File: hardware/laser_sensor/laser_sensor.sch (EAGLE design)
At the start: 11 parts, among them IC1 NE555D, J1 B4B-XH-A(LF)(SN)

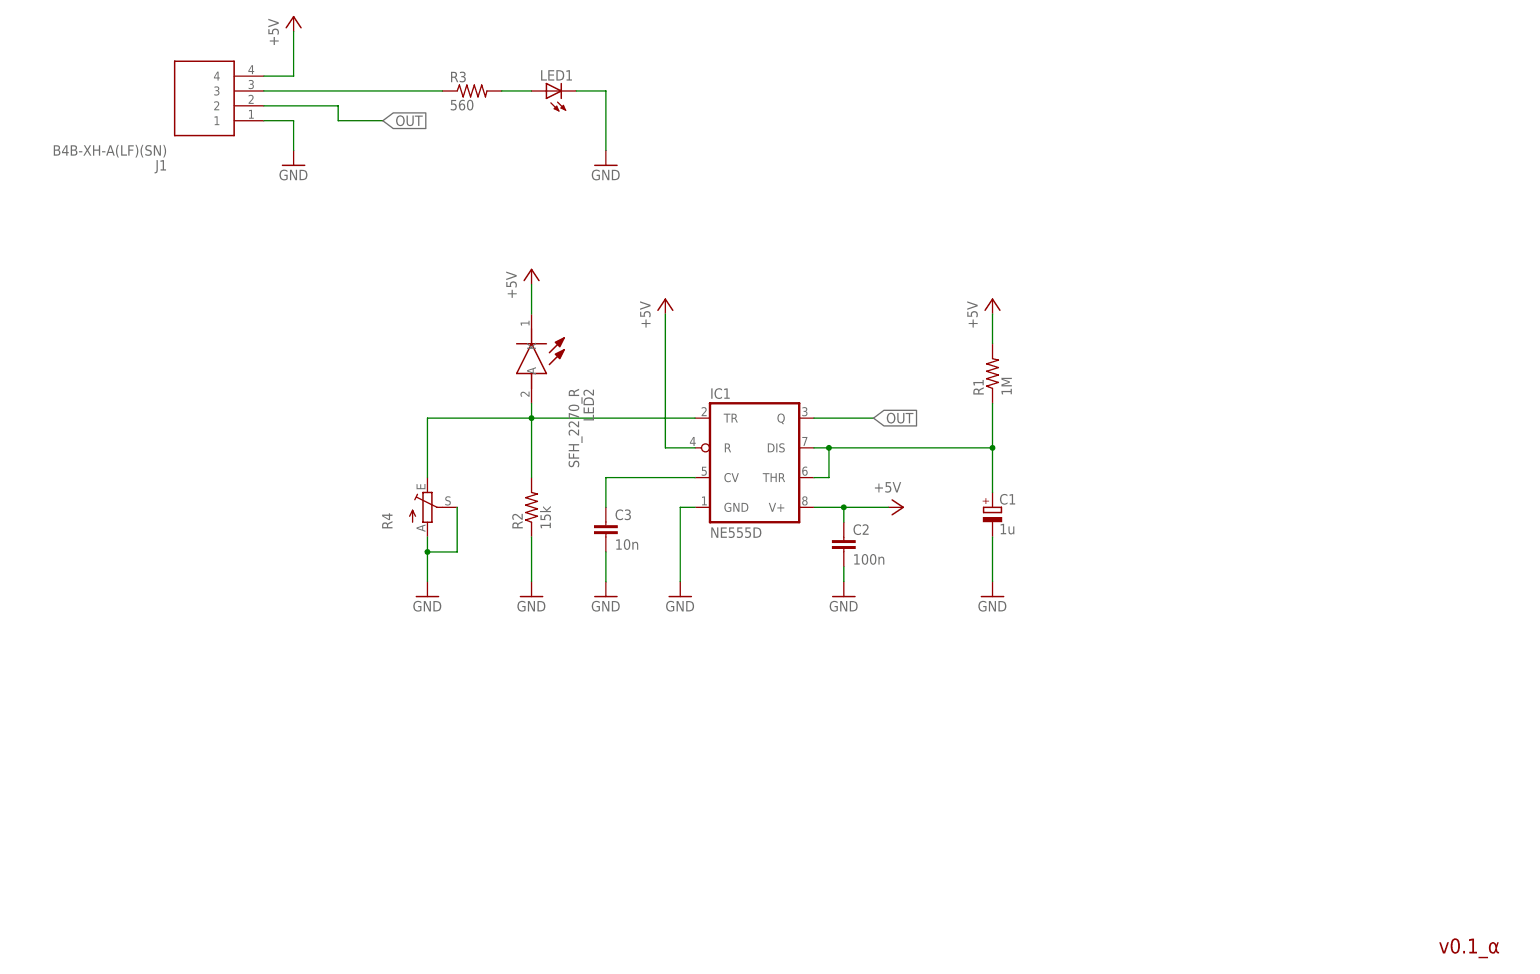
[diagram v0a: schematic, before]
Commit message: sensor redesign
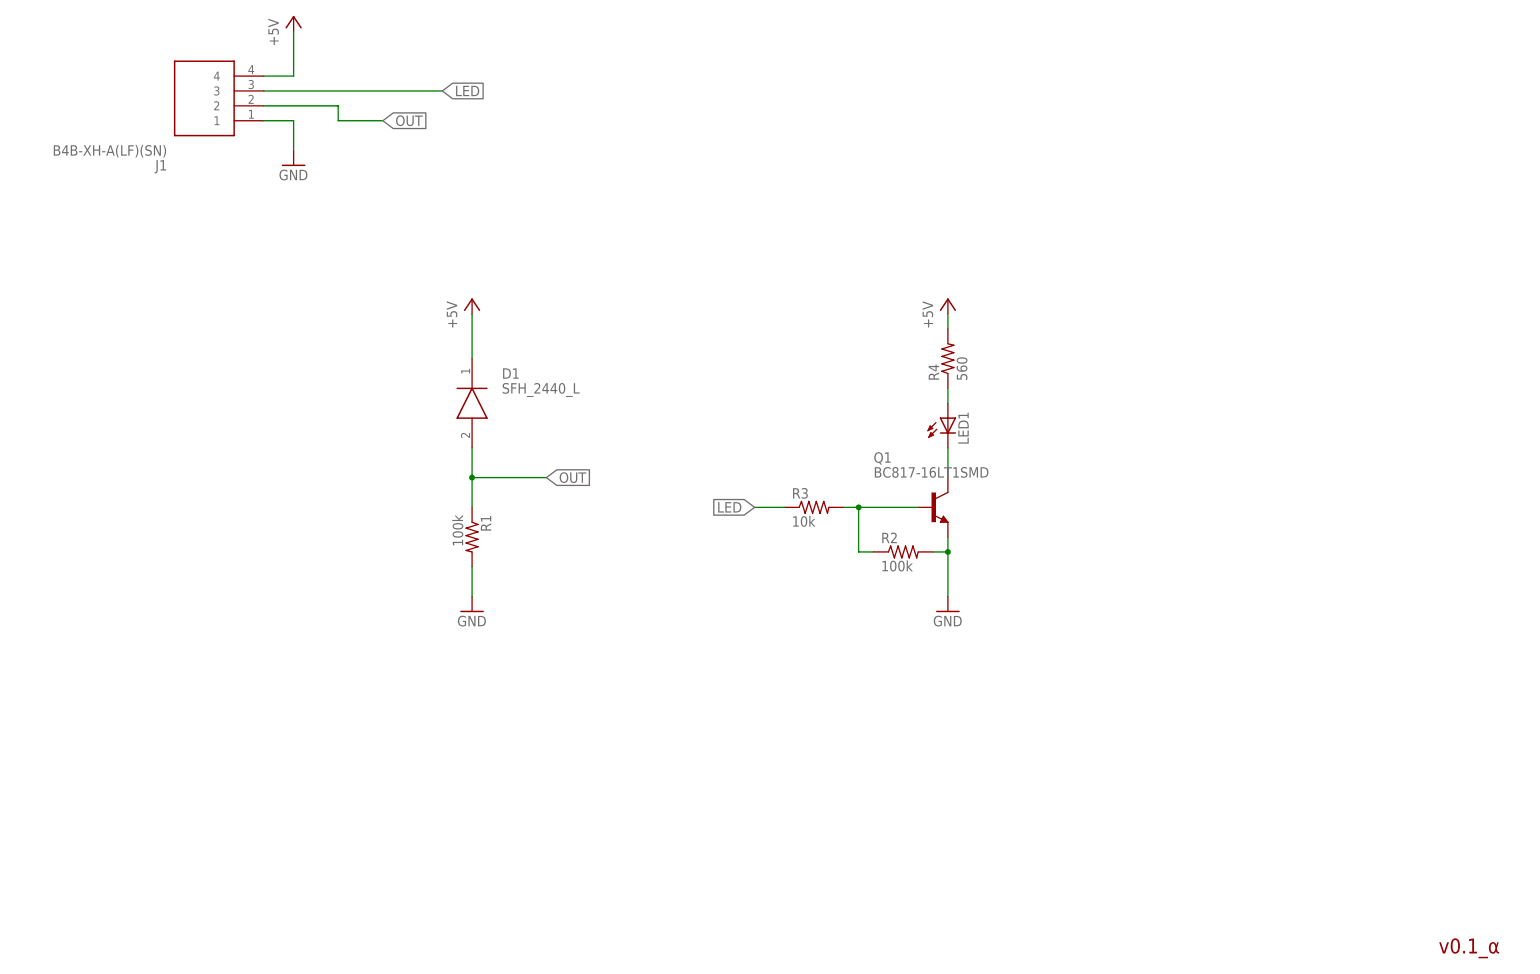
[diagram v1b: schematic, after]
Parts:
- removed C1: 1u, rcl:CPOL-EU153CLV-0405
- removed C2: 100n, rcl:C-EUC0603K
- removed C3: 10n, rcl:C-EUC0805K
- removed IC1: NE555D, linear:NE555D
- removed LED2: SFH_2270_R, SFH_2270_R:SFH_2270_R
- added D1: SFH_2440_L, SFH_2440_L:SFH_2440_L
- added Q1: BC817-16LT1SMD, transistor-npn:BC817-16LT1SMD
- R1: value 1M -> 100k; device resistor:R-US_M0805 -> rcl:R-US_R0603
- R2: value 15k -> 100k; device resistor:R-US_M0805 -> rcl:R-US_R0603
- R3: value 560 -> 10k; device resistor:R-US_M0805 -> rcl:R-US_R0603
- R4: value (none) -> 560; device pot:TRIM_EU-B64Y -> rcl:R-US_R0603
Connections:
- net N$2 renamed LED
- removed net N$4: C3.1, IC1.CV
- removed net N$5: LED1.A, R3.2
- new net N$2: LED1.C, Q1.C
- net +5V: now also D1.ANODE, R4.2; no longer C2.1, IC1.R, IC1.V+, LED2.K, R1.2
- net GND: now also Q1.E, R1.2, R2.2; no longer C1.-, C2.2, C3.2, IC1.GND, LED1.C, R2.1, R4.A, R4.S
- net N$1: now also LED1.A, R4.1; no longer C1.+, IC1.DIS, IC1.THR, R1.1
- net N$3: now also Q1.B, R2.1, R3.2; no longer IC1.TR, LED2.A, R2.2, R4.E
- net OUT: now also D1.CATHODE, R1.1; no longer IC1.Q
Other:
- moved on the sheet: LED1, R1, R2, R3
